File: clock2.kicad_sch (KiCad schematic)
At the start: 37 parts, among them CN1 PJ-327A 5JJ, CN2 PJ-327A 5JJ, SW1 SSSS811101, U1 NE555D, U2 NE555D, U3 TC-6615-9.0-160G, U4 NE555D, U5 XL74LS04, U6 XL74LS08, U7 XL74LS32, U8 RM063-105(1M)

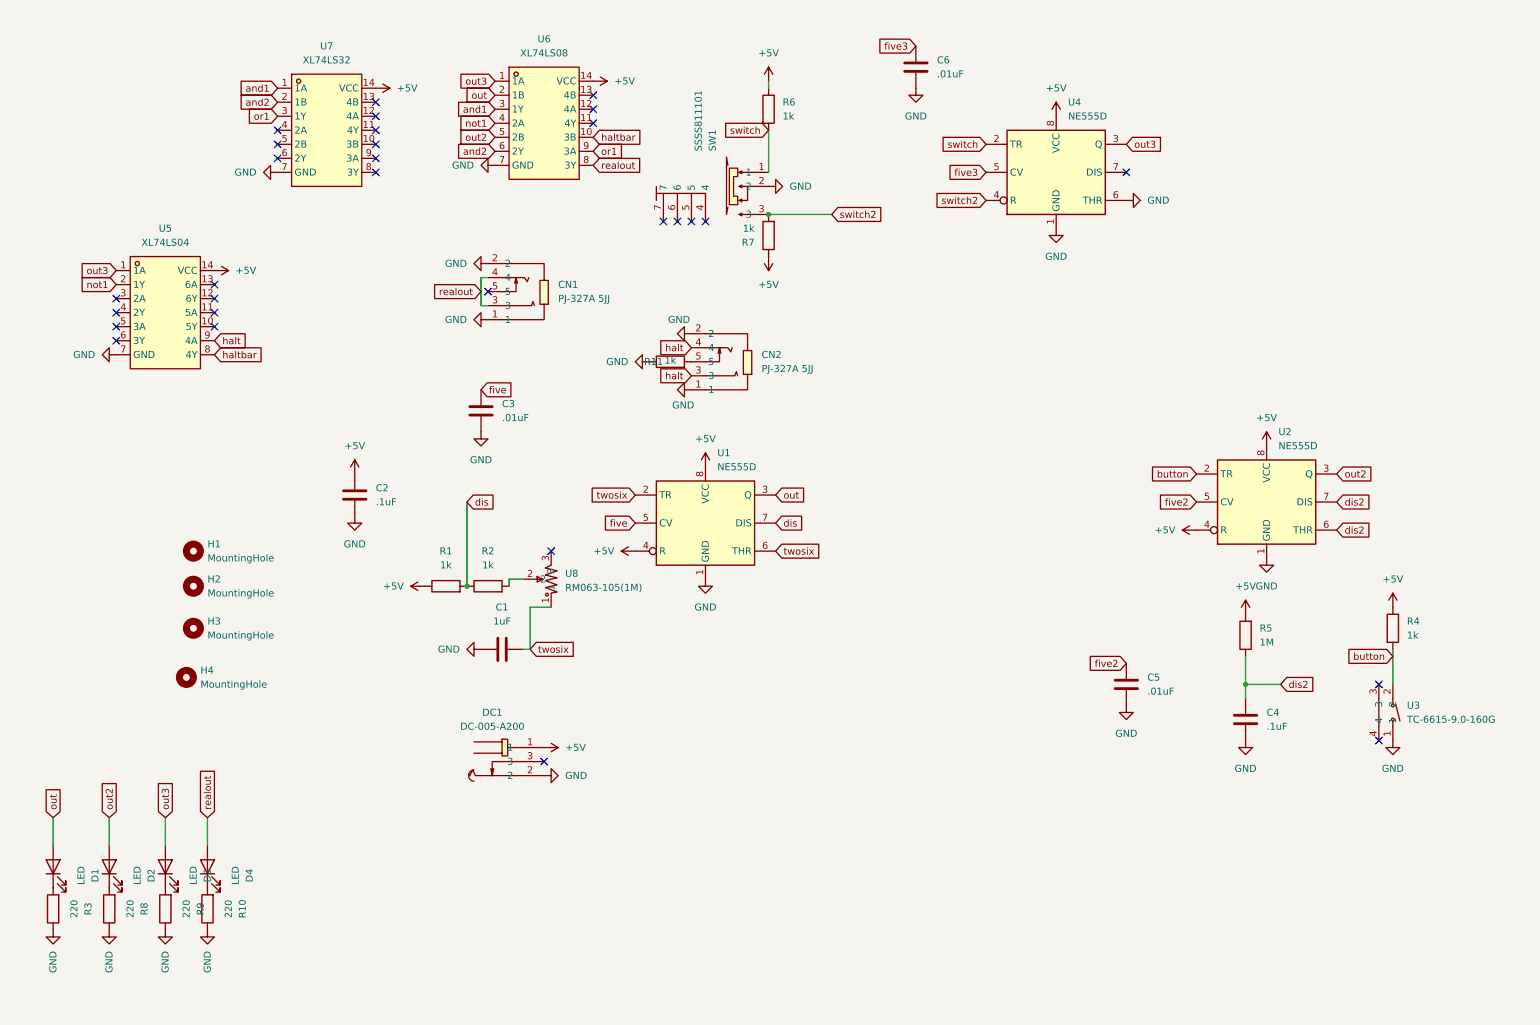
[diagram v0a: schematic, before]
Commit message: v1 finalized
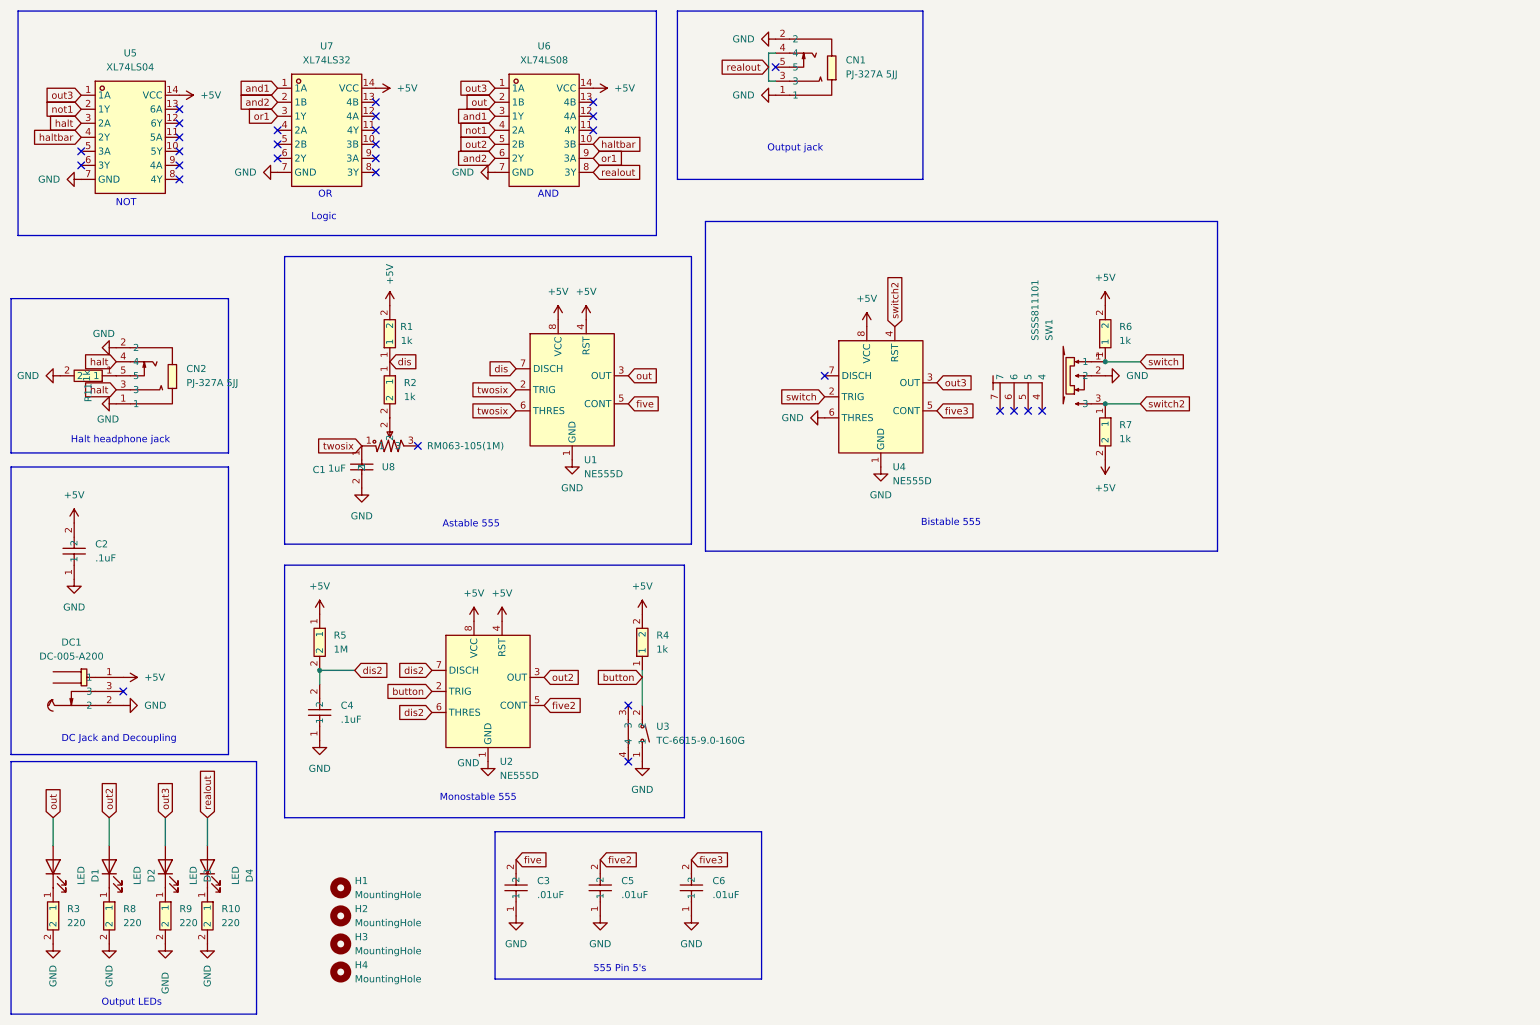
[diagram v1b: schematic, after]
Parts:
- C1: footprint Capacitor_SMD:C_0805_2012Metric_Pad1.18x1.45mm_HandSolder -> easyeda2kicad:C0805; symbol Device:C -> easyeda2kicad:CL21B105KBFNNNE; LCSC Part (none) -> C28323
- C2, C4: footprint Capacitor_SMD:C_0805_2012Metric_Pad1.18x1.45mm_HandSolder -> easyeda2kicad:C0805; symbol Device:C -> easyeda2kicad:CC0805KRX7R9BB104; LCSC Part (none) -> C49678
- C3, C5, C6: footprint Capacitor_SMD:C_0805_2012Metric_Pad1.18x1.45mm_HandSolder -> easyeda2kicad:C0805; symbol Device:C -> easyeda2kicad:CC0805KRX7R9BB103; LCSC Part (none) -> C83170
- R1, R11, R2, R4, R6, R7: footprint Resistor_SMD:R_0805_2012Metric_Pad1.20x1.40mm_HandSolder -> easyeda2kicad:R0805; symbol Device:R -> easyeda2kicad:RC0805FR-071KL; LCSC Part (none) -> C95781
- R10, R3, R8, R9: footprint Resistor_SMD:R_0805_2012Metric_Pad1.20x1.40mm_HandSolder -> easyeda2kicad:R0805; symbol Device:R -> easyeda2kicad:0805W8F2200T5E; LCSC Part (none) -> C17557
- R5: footprint Resistor_SMD:R_0805_2012Metric_Pad1.20x1.40mm_HandSolder -> easyeda2kicad:R0805; symbol Device:R -> easyeda2kicad:RC0805FR-071ML; LCSC Part (none) -> C107700
- U1, U2, U4: footprint Package_SO:SOIC-8_3.9x4.9mm_P1.27mm -> easyeda2kicad:SOIC-8_L4.9-W3.9-P1.27-LS6.0-BL; symbol Timer:NE555D -> easyeda2kicad:NE555DR; LCSC Part (none) -> C7593
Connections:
- net +5V: now also C2.2, R1.2, R4.2, R5.1, R6.2, R7.2; no longer C2.1, R1.1, R4.1, R5.2, R6.1, R7.1
- net GND: now also C1.2, C2.1, C3.1, C4.1, C5.1, C6.1, R10.2, R11.2, R3.2, R8.2, R9.2; no longer C1.1, C2.2, C3.2, C4.2, C5.2, C6.2, R10.1, R11.1, R3.1, R8.1, R9.1
- net button: now also R4.1; no longer R4.2
- net dis: now also R1.1; no longer R1.2
- net dis2: now also C4.2, R5.2; no longer C4.1, R5.1
- net five: now also C3.2; no longer C3.1
- net five2: now also C5.2; no longer C5.1
- net five3: now also C6.2; no longer C6.1
- net halt: now also U5.3 (2A); no longer U5.9 (4A)
- net haltbar: now also U5.4 (2Y); no longer U5.8 (4Y)
- net switch: now also R6.1; no longer R6.2
- net switch2: now also R7.1; no longer R7.2
- net twosix: now also C1.1; no longer C1.2
- net at D3.1 (K): now also R9.1; no longer R9.2
- net at CN2.5: now also R11.1; no longer R11.2
- net at D4.1 (K): now also R10.1; no longer R10.2
- net at D1.1 (K): now also R3.1; no longer R3.2
- net at D2.1 (K): now also R8.1; no longer R8.2
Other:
- note added: "555 Pin 5's"
- note added: "AND"
- note added: "Astable 555"
- note added: "Bistable 555"
- note added: "DC Jack and Decoupling"
- note added: "Halt headphone jack"
- note added: "Logic"
- note added: "Monostable 555"
- note added: "NOT"
- note added: "OR"
- note added: "Output LEDs"
- note added: "Output jack"
- moved on the sheet: CN1, CN2, DC1, H1, H2, H3, H4, SW1, U3, U5, U6, U8
